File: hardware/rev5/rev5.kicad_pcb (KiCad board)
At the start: 2 copper layers, 39.2 x 44.1 mm, 25 parts, among them J3 Conn_02x03_Odd_Even, J4 Conn_01x05, J5 Conn_01x02

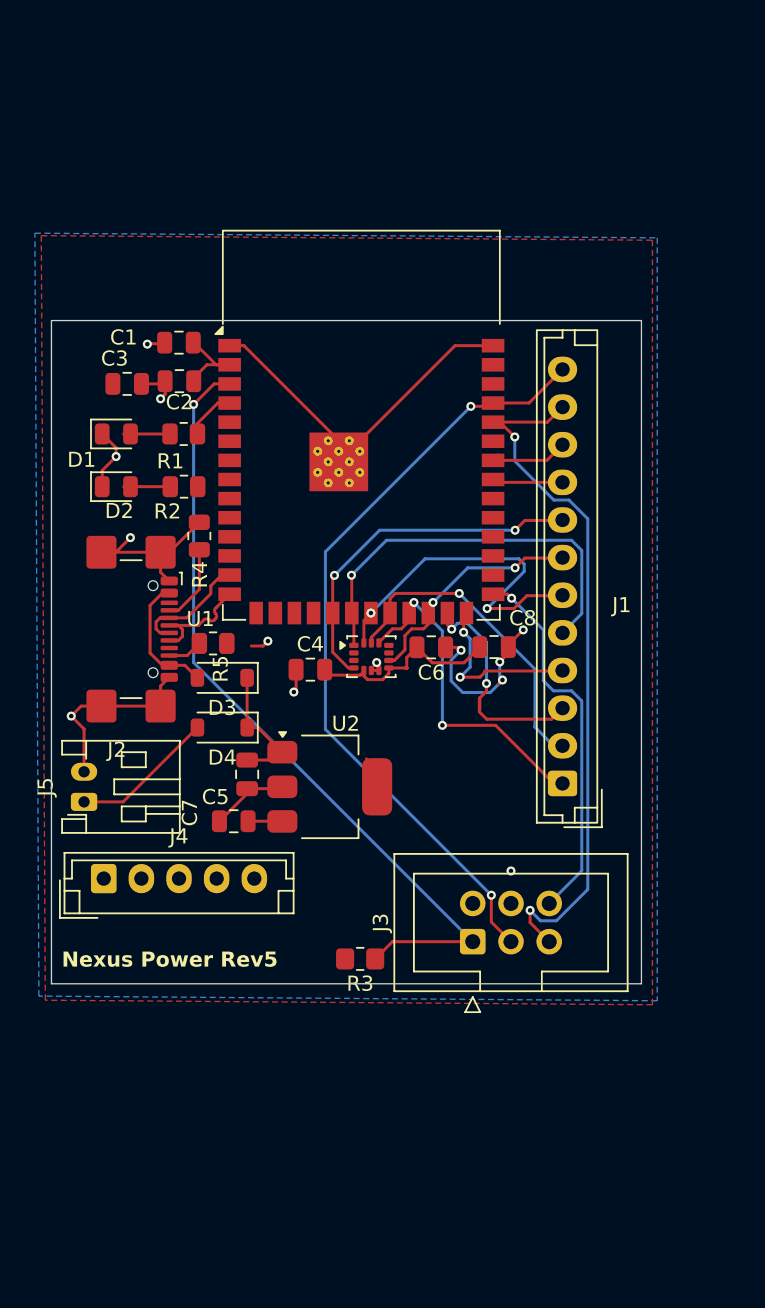
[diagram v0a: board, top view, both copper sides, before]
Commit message: Rev 5 changes
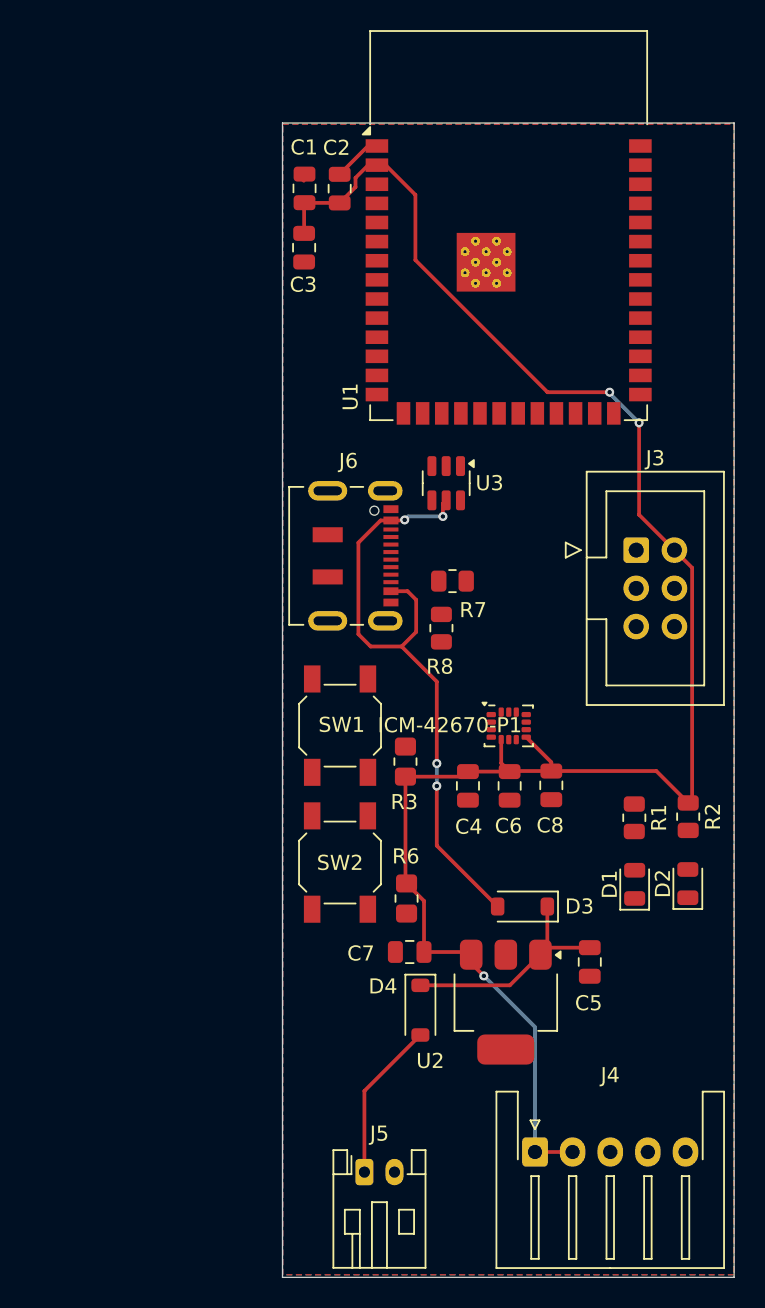
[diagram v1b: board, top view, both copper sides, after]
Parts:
- removed J1: ~, Connector_JST:JST_EH_B12B-EH-A_1x12_P2.50mm_Vertical
- removed J2: ~, Connector_USB:USB_C_Receptacle_GCT_USB4110
- removed R4, R5: 5.1k, Resistor_SMD:R_0805_2012Metric
- added J6: USB_C_Receptacle_USB2.0_16P, Connector_USB:USB_C_Receptacle_JAE_DX07S016JA1R1500, F.Cu at (138.2, 90.7)
- added R6: 5k, Resistor_SMD:R_0805_2012Metric_Pad1.20x1.40mm_HandSolder, F.Cu at (142.3, 113.5)
- added R7: 5.1k, Resistor_SMD:R_0805_2012Metric, F.Cu at (145.3, 92.4)
- added R8: 5.1k, Resistor_SMD:R_0805_2012Metric, F.Cu at (144.6, 95.5)
- added SW1: SW_Push, Button_Switch_SMD:SW_SPST_SKQG_WithStem, F.Cu at (137.9, 102.0)
- added SW2: SW_Push, Button_Switch_SMD:SW_SPST_SKQG_WithStem, F.Cu at (137.9, 111.1)
- added U3: USBLC6-2SC6, Package_TO_SOT_SMD:SOT-23-6, F.Cu at (144.9, 85.9)
- J4: footprint Connector_JST:JST_EH_B5B-EH-A_1x05_P2.50mm_Vertical -> Connector_JST:JST_XH_S5B-XH-A-1_1x05_P2.50mm_Horizontal
- moved D2 46.2 mm to (161.0, 112.5), turned to 90 degrees
- moved D1 45.6 mm to (157.4, 112.5), turned to 90 degrees
- moved R2 40.0 mm to (161.0, 108.0), turned to -90 degrees
- moved R1 39.3 mm to (157.4, 108.1), turned to -90 degrees
- moved J4 33.9 mm to (150.8, 130.3)
- moved J5 30.8 mm to (139.5, 131.6), turned to 0 degrees
- moved J3 28.2 mm to (157.5, 90.3), turned to 0 degrees
- moved C5 25.9 mm to (154.5, 117.7)
- moved D3 25.1 mm to (150.0, 114.0)
- moved D4 22.9 mm to (143.2, 120.9), turned to -90 degrees
- moved U2 18.5 mm to (148.9, 120.3), turned to -90 degrees
- moved C2 16.6 mm to (137.8, 66.3), turned to 90 degrees
- moved U1 16.5 mm to (149.1, 68.7)
- moved C3 14.8 mm to (135.5, 70.2), turned to -90 degrees
- moved C7 14.6 mm to (142.5, 117.0)
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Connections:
- net /IO0 renamed /BOOT
- J4 pad 1: /VDD -> +3.3V
- J4 pad 2: /VCC -> +3.3V
- R3 pad 1: /EN -> +3.3V
- R3 pad 2: +3.3V -> /EN
- U1 pad 33: /GPIO10 -> unconnected-(U1-IO40-Pad33)
- U1 pad 34: /GPIO9 -> unconnected-(U1-IO41-Pad34)
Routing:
- net +3.3V: track 21.6 -> 120.1 mm, vias 0 -> 3
- net GND: track 79.4 -> 3.28 mm, vias 13 -> 0
- net /EN: track 53.3 -> 0.00 mm, vias 1 -> 0
- net /TX: track 51.8 -> 0.00 mm, vias 2 -> 0
- net /RX: track 47.1 -> 0.00 mm, vias 2 -> 0
- net +5V_USB: track 8.61 -> 42.1 mm, vias 0 -> 4
- net /MISO: track 30.3 -> 0.00 mm, vias 1 -> 0
- net /BOOT: track 25.1 -> 0.00 mm, vias 1 -> 0
- net /INT1 Gyro: track 23.2 -> 0.00 mm, vias 2 -> 0
- net /MOSI: track 22.1 -> 0.00 mm, vias 2 -> 0
- net /CS Gyro: track 22.1 -> 0.00 mm, vias 2 -> 0
- net /SCLK: track 21.8 -> 0.00 mm, vias 1 -> 0
- net /INT2 Gyro: track 15.8 -> 0.00 mm, vias 2 -> 0
- net /HX711 PDSCK: track 15.7 -> 0.00 mm, vias 2 -> 0
- net /HX711 DOUT: track 11.4 -> 0.00 mm, vias 2 -> 0
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- added copper zone on F.Cu, net GND
- removed copper zone on F.Cu, net +3.3V
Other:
- board size 39.2 x 44.1 mm -> 30 x 76.7 mm
- board text removed: "Nexus Power Rev5"
